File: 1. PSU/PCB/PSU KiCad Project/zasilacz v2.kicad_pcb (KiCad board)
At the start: 2 copper layers, 47 x 51 mm, 23 parts, among them J1 USB_B, J2 Conn_01x04, J3 Conn_01x04, J4 Conn_01x04, J5 Conn_01x04, J6 Conn_01x04, U1 MIC4576, U2 TC7660H

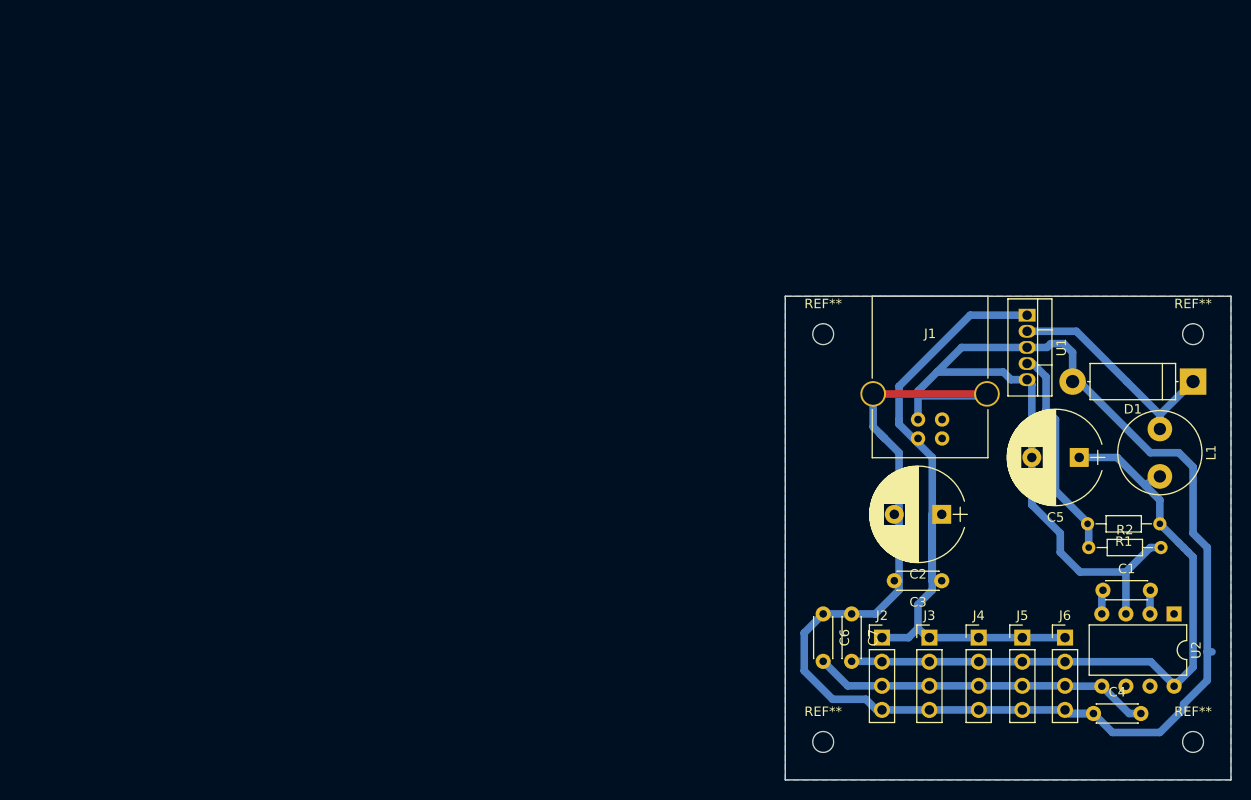
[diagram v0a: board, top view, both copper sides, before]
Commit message: Amiga rulez
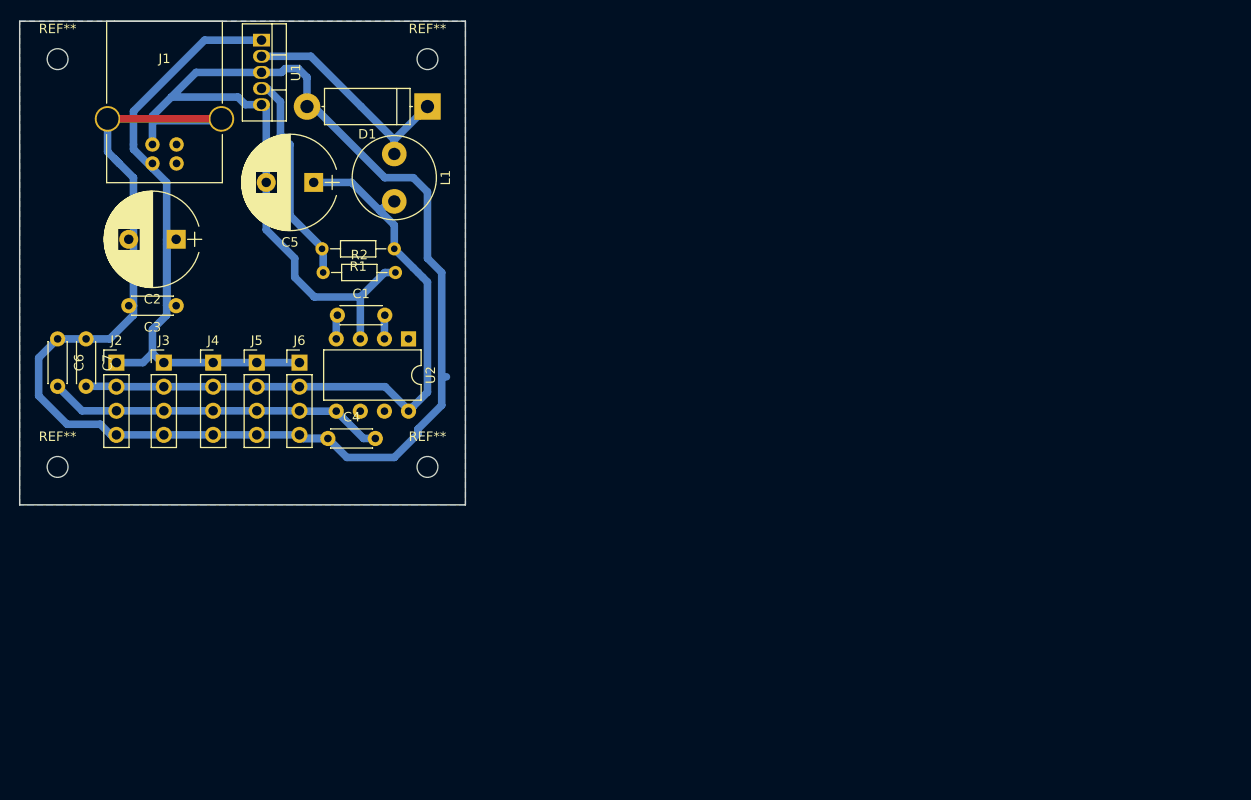
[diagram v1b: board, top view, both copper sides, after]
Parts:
- moved J4 85.8 mm to (62.7, 55.0)
- moved C1 85.8 mm to (75.8, 50.0)
- moved C2 85.8 mm to (58.8, 42.0)
- moved C3 85.8 mm to (58.8, 49.0)
- moved C4 85.8 mm to (74.8, 63.0)
- moved C5 85.8 mm to (73.3, 36.0)
- moved C6 85.8 mm to (46.3, 52.5)
- moved C7 85.8 mm to (49.3, 52.5)
- moved D1 85.8 mm to (85.3, 28.0)
- moved J1 85.8 mm to (56.3, 34.0)
- moved J2 85.8 mm to (52.5, 55.0)
- moved J3 85.8 mm to (57.5, 55.0)
- moved J5 85.8 mm to (67.3, 55.0)
- moved J6 85.8 mm to (71.8, 55.0)
- moved L1 85.8 mm to (81.8, 33.0)
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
